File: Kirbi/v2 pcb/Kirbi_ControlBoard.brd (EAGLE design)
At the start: 66 x 56 mm, 72 parts, among them U1 PCA9306_LSSOP, U2 TEENSY_3.6_DIL, U5 LM393-8-SOIC, U6 AP2114H-1.8TRG1, U7 AP2114H-3.3TRG1

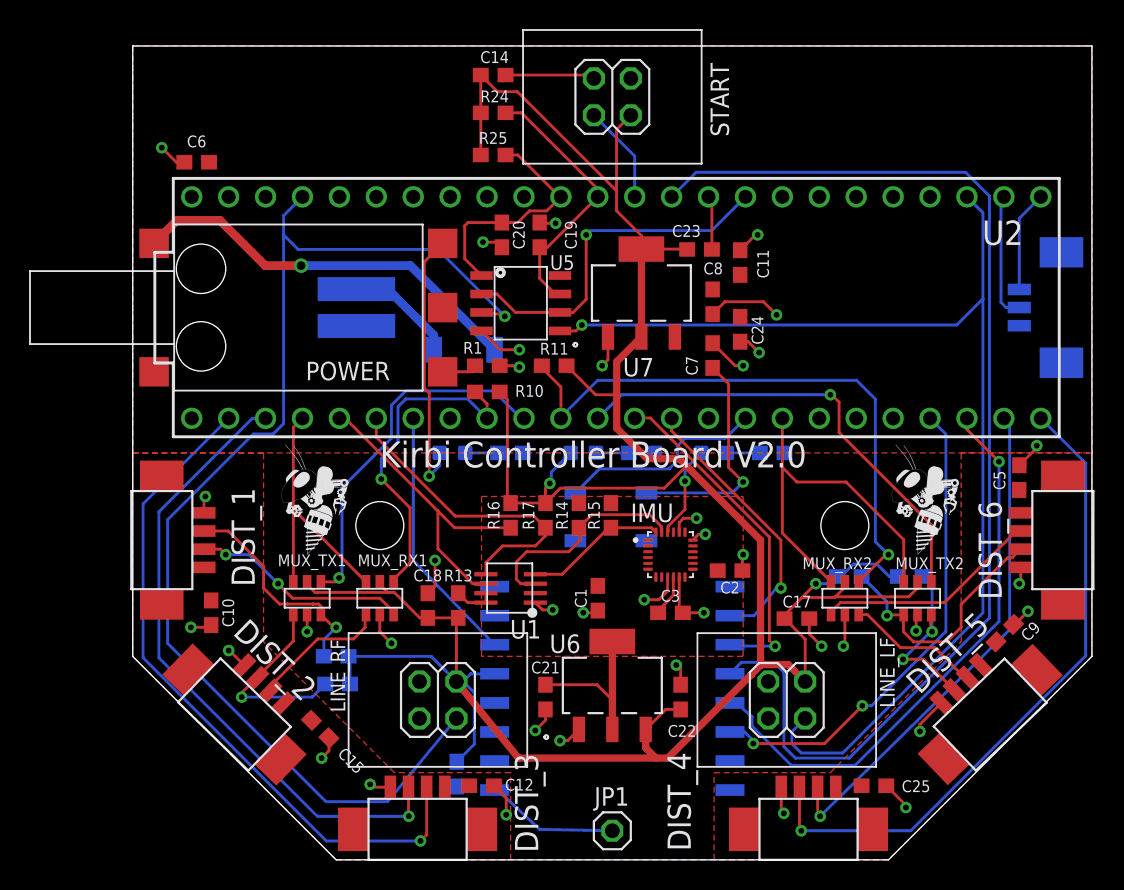
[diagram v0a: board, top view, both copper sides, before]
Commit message: Fixed Clearances  - Changed DRC
Fixed Clearance  - Changed DRC (JLCPCB Layer 2)
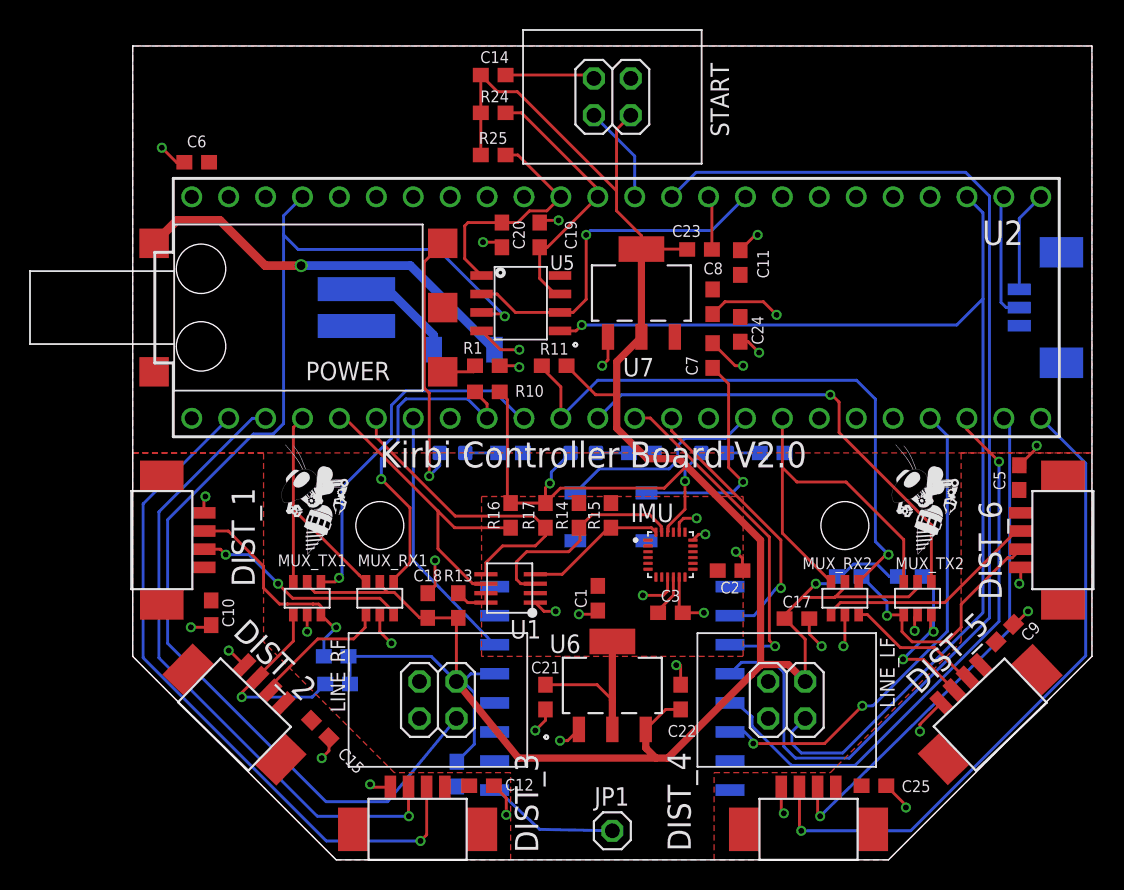
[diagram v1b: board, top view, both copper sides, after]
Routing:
- net GND: track 82.6 -> 83.8 mm
